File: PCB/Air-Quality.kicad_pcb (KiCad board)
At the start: 2 copper layers, 22 x 52 mm, 17 parts, among them J1 Conn_01x07_Female, SW1 SW_Push, SW2 SW_SPST, U1 Pico

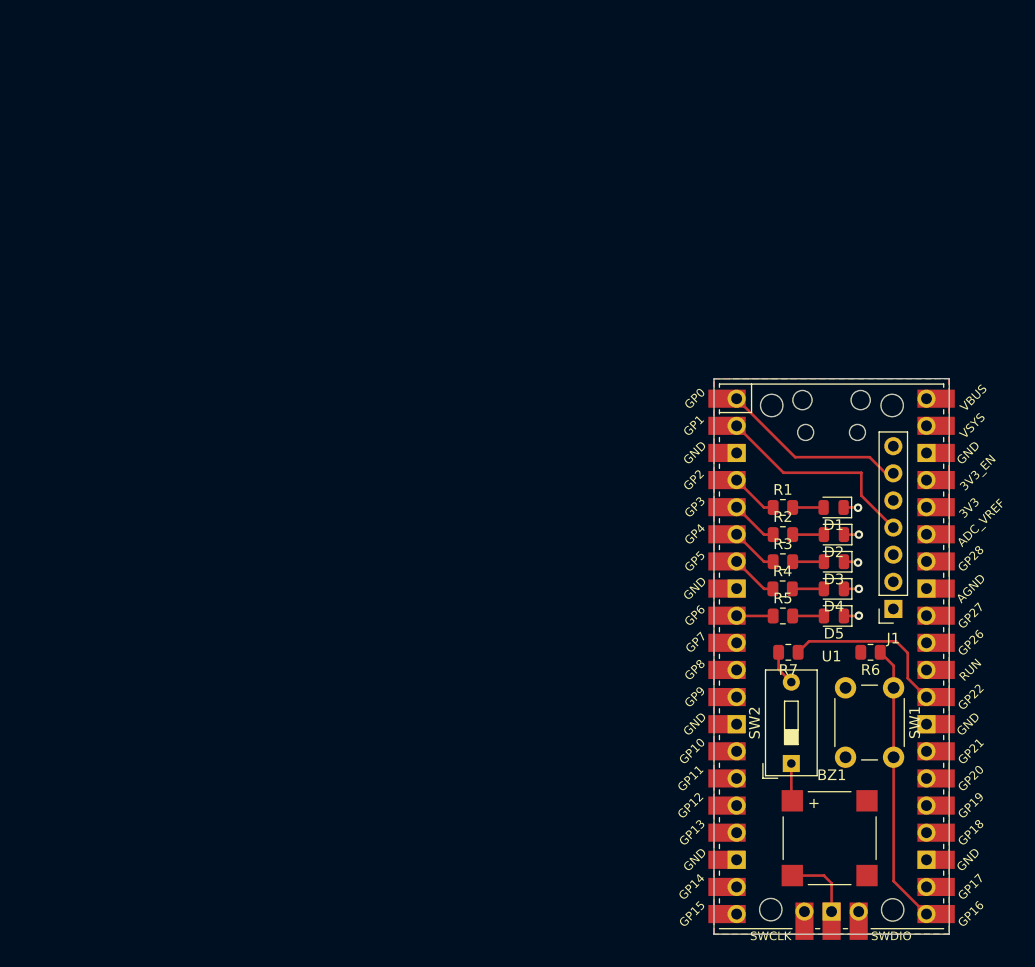
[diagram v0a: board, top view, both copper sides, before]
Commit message: Version 3 for friends.
Seeeduino
New Sensor
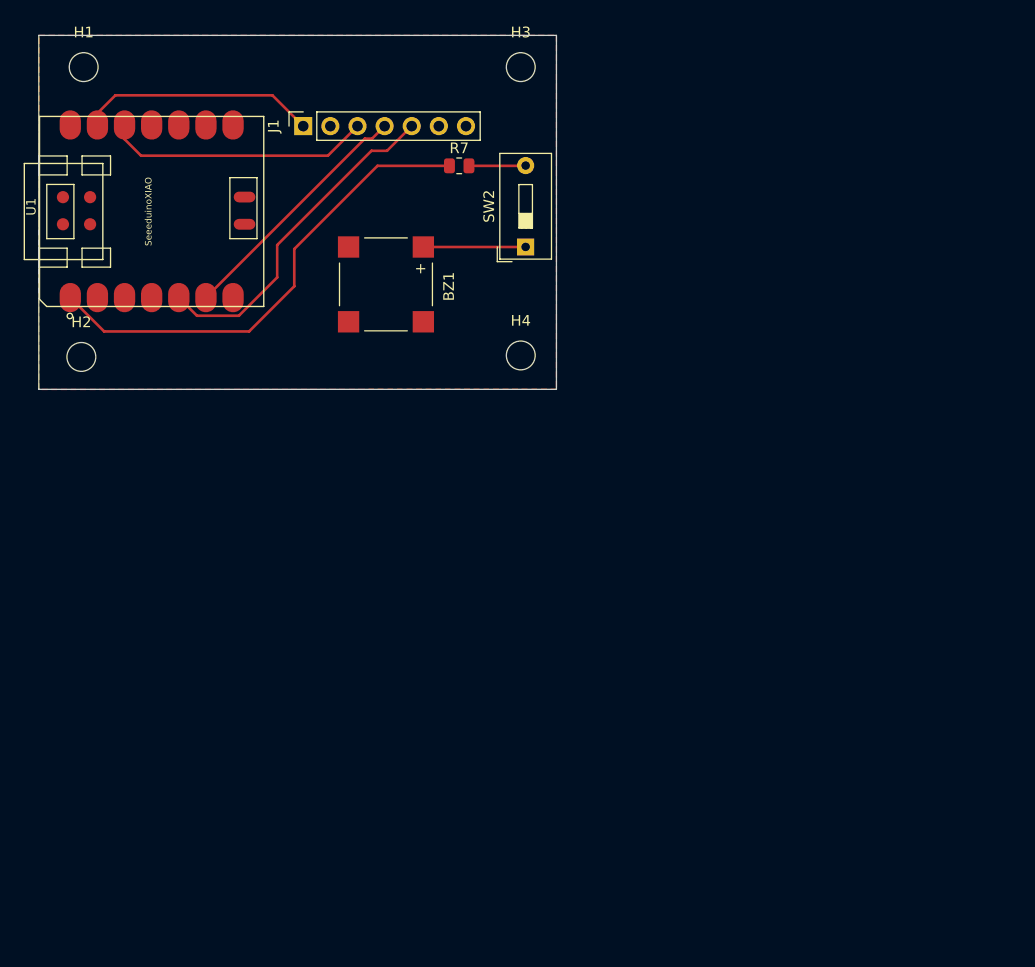
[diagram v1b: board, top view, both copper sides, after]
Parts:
- removed D1, D2, D3, D4, D5: LED, LED_SMD:LED_0805_2012Metric
- removed R1, R2, R3, R4, R5: 220 Ohm, Resistor_SMD:R_0805_2012Metric
- removed R6: 10kOhm, Resistor_SMD:R_0805_2012Metric
- removed SW1: SW_Push, Button_Switch_THT:SW_PUSH_6mm
- added H1: MountingHole, MountingHole:MountingHole_2.7mm_M2.5_ISO14580, F.Cu at (116.8, 33.1)
- added H2: MountingHole, MountingHole:MountingHole_2.7mm_M2.5_ISO14580, F.Cu at (116.5, 60.2)
- added H3: MountingHole, MountingHole:MountingHole_2.7mm_M2.5_ISO14580, F.Cu at (157.7, 33.1)
- added H4: MountingHole, MountingHole:MountingHole_2.7mm_M2.5_ISO14580, F.Cu at (157.7, 60.1)
- U1: value Pico -> SeeeduinoXIAO; footprint MCU_RaspberryPI_and_Board:RPi_Pico_SMD_TH -> Seeeduino XIAO KICAD:Seeeduino XIAO-MOUDLE14P-2.54-21X17.8MM
- moved J1 71.4 mm to (137.3, 38.6), turned to 90 degrees
- moved BZ1 66.4 mm to (145.1, 53.5), turned to 270 degrees
- moved U1 62.5 mm to (133.6, 55.5), turned to 90 degrees
- moved R7 55.0 mm to (151.9, 42.4), turned to 0 degrees
- moved SW2 54.4 mm to (158.2, 49.9)
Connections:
- J1 pad 1: +3V3 -> GND
- J1 pad 3: GND -> +3V3
- J1 pad 5: Net-(J1-Pad5) -> /SDA
- J1 pad 6: /SDA -> Net-(J1-Pad6)
- U1 pad 1: /SDA -> Net-(R7-Pad1)
- U1 pad 12: Net-(U1-Pad12) -> +3V3
- U1 pad 16: Net-(U1-Pad16) -> GND
- U1 pad 18: GND -> Net-(U1-Pad18)
- U1 pad 2: /SCL -> Net-(U1-Pad2)
- U1 pad 20: Net-(U1-Pad20) -> GND
- U1 pad 3: GND -> Net-(U1-Pad3)
- U1 pad 5: Net-(R2-Pad1) -> /SDA
- U1 pad 6: Net-(R3-Pad1) -> /SCL
- U1 pad 8: GND -> Net-(U1-Pad8)
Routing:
- net Net-(R7-Pad1): track 16.0 -> 45.3 mm
- net Net-(R6-Pad1): track 26.3 -> 0.00 mm
- net +3V3: track 0.00 -> 24.9 mm
- net /SDA: track 17.6 -> 31.6 mm
- net GND: track 13.6 -> 22.3 mm, vias 5 -> 0
- net Net-(BZ1-Pad1): track 3.63 -> 9.58 mm
- net Net-(U1-Pad4): track 4.48 -> 0.00 mm
- net Net-(R3-Pad1): track 4.48 -> 0.00 mm
- net Net-(R2-Pad1): track 4.48 -> 0.00 mm
- net Net-(U1-Pad7): track 4.46 -> 0.00 mm
- net /SCL: track 19.9 -> 23.4 mm
- net Net-(U1-Pad9): track 3.43 -> 0.00 mm
- net Net-(D4-Pad2): track 2.95 -> 0.00 mm
- net Net-(D3-Pad2): track 2.93 -> 0.00 mm
- net Net-(D5-Pad2): track 2.93 -> 0.00 mm
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- added copper zone on F.Cu, net GND
- removed copper zone on F.Cu, net +3V3
- removed copper zone on B.Cu, net GND
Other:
- board size 22 x 52 mm -> 48.5 x 33.1 mm
